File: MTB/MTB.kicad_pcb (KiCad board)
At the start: 2 copper layers, 45 parts, among them J1 BAT_CONN

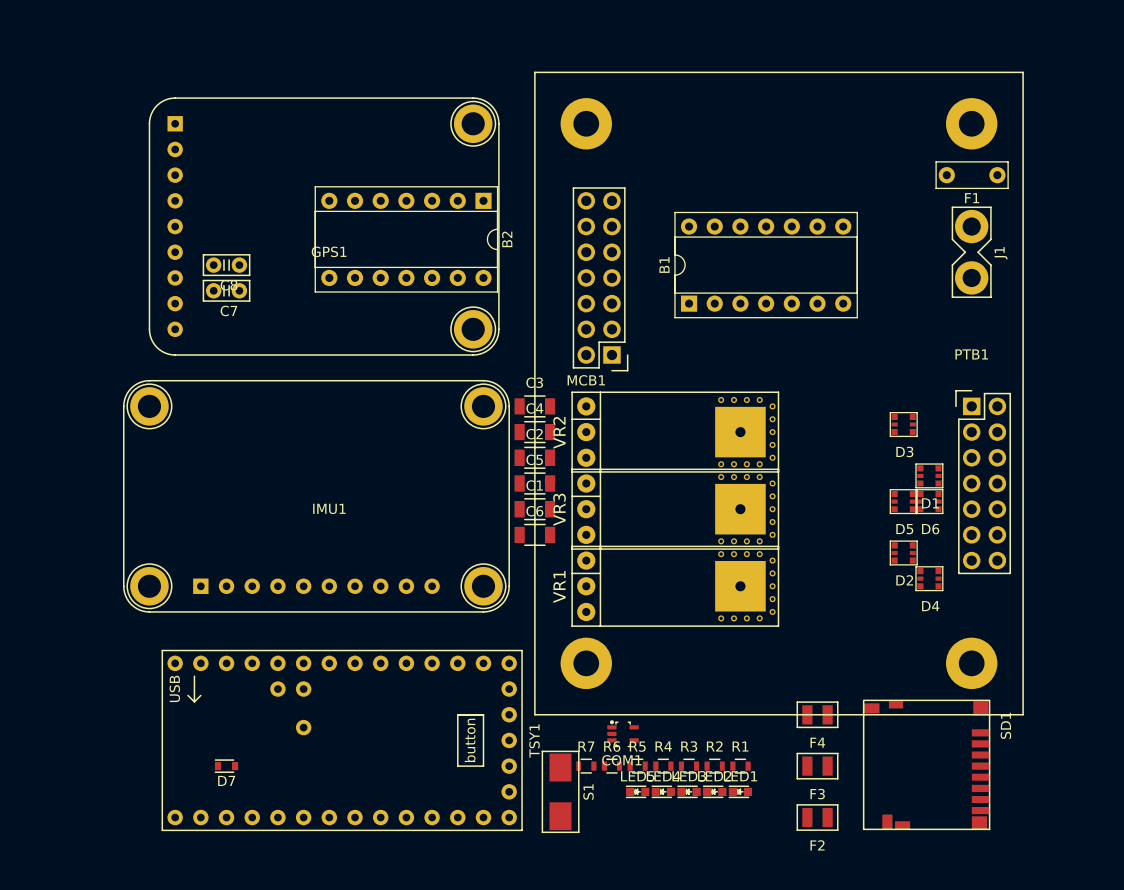
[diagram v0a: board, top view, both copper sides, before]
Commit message: finished motherboard
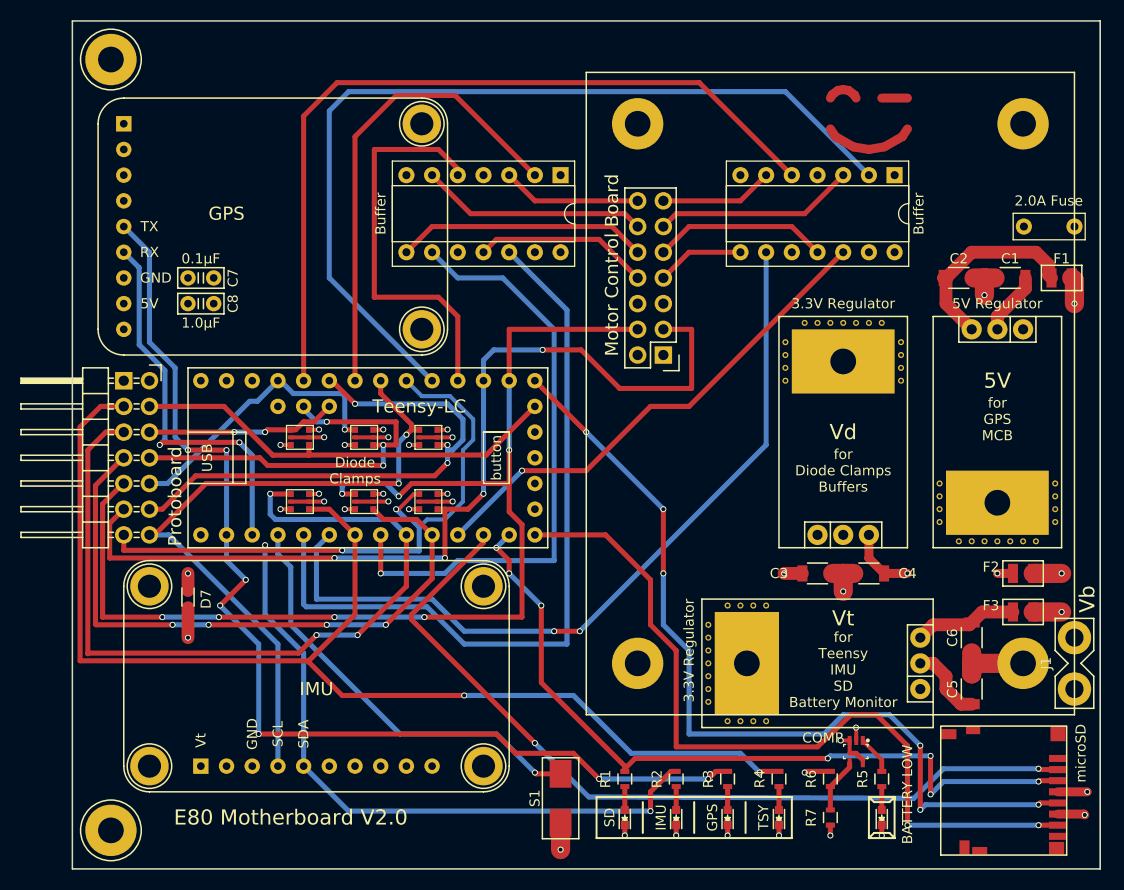
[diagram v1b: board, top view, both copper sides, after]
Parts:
- removed F4: 0.35A Fuse, MTB_footprints:1206
- removed PTB1: Protoboard, Pin_Headers:Pin_Header_Straight_2x07
- removed VR1: 5V_Regulator, MTB_footprints:VREG
- removed VR2, VR3: 3.3V_Regulator, MTB_footprints:VREG
- added 2.0A Fuse: 2.0A Fuse, Capacitors_THT:C_Disc_D7.0mm_W2.5mm_P5.00mm, F.Cu at (215.9, 83.8)
- added 3.3V Regulator: 3.3V_Regulator, MTB_footprints:VREG, F.Cu at (193.0, 114.3)
- added 3.3V Regulator: 3.3V_Regulator, MTB_footprints:VREG, F.Cu at (200.7, 127.0)
- added 5V Regulator: 5V_Regulator, MTB_footprints:VREG, F.Cu at (208.3, 94.0)
- added Protoboard: Protoboard, MTB_footprints:PTB_CONN, F.Cu at (124.5, 99.1)
- added T1: TEST_HOLE, MCB_footprints:TESTPOINT_LARGE, F.Cu at (120.7, 67.3)
- added T2: TEST_HOLE, MCB_footprints:TESTPOINT_LARGE, F.Cu at (120.7, 143.5)
- BATTERY LOW: renamed from LED5
- Buffer: renamed from B2; value Buffer -> Buffer2
- F1: value 2.0A Fuse -> .35A Fuse; footprint Capacitors_THT:C_Disc_D7.0mm_W2.5mm_P5.00mm -> MTB_footprints:1206
- F2: value 0.35A Fuse -> .35A Fuse
- F3: value 0.5A Fuse -> .5A Fuse
- Motor Control Board: renamed from MCB1
- moved D6 62.6 mm to (138.4, 105.4)
- moved D1 62.3 mm to (138.4, 111.8)
- moved D5 53.7 mm to (144.8, 105.4)
- moved D2 53.6 mm to (144.8, 111.8)
- moved C1 52.3 mm to (209.6, 88.9), turned to 180 degrees
- moved D4 51.5 mm to (151.1, 105.4)
- moved C5 47.7 mm to (205.7, 129.5), turned to 90 degrees
- moved D3 47.6 mm to (151.1, 111.8)
- moved C2 45.5 mm to (204.5, 88.9)
- moved C6 44.4 mm to (205.7, 124.5), turned to 270 degrees
- moved J1 41.9 mm to (215.9, 127.0), turned to 270 degrees
- moved Buffer 40.7 mm to (198.1, 78.7)
- moved C4 35.9 mm to (195.6, 118.1), turned to 180 degrees
- moved C3 32.5 mm to (190.5, 118.1)
- moved F2 31.5 mm to (210.8, 118.1), turned to 180 degrees
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- renumbered B1 to Buffer, COM1 to COMP, GPS1 to GPS, LED3 to GPS, IMU1 to IMU, LED2 to IMU, LED1 to SD, LED4 to TSY, TSY1 to Teensy-LC, SD1 to microSD
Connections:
- Buffer pad 14: Vt -> Vd (x2)
- Buffer pad 11: /2A -> /4A
- Buffer pad 12: 2AT -> 4AT
- Buffer pad 2: 8AT -> 6AT
- Buffer pad 3: /8A -> /6A
- Buffer pad 5: 6AT -> 8AT
- Buffer pad 6: /6A -> /8A
- Buffer pad 8: /4A -> /2A
- Buffer pad 9: 4AT -> 2AT
- C1 pad 1: Net-(C1-Pad1) -> +5V
- C2 pad 1: +5V -> Net-(C2-Pad1)
- C3 pad 1: Net-(C3-Pad1) -> Vd
- C4 pad 1: Vt -> Net-(C4-Pad1)
- C5 pad 1: Net-(C5-Pad1) -> Vt
- C6 pad 1: Vd -> Net-(C6-Pad1)
- F1 pad 1: Vm -> Vb
- F1 pad 2: Net-(F1-Pad2) -> Net-(C2-Pad1)
- F2 pad 1: Vm -> Vb
- F2 pad 2: Net-(C1-Pad1) -> Net-(C4-Pad1)
- F3 pad 1: Vm -> Vb
- F3 pad 2: Net-(C3-Pad1) -> Net-(C6-Pad1)
- J1 pad 1: Vm -> Vb
- Motor Control Board pad 3: Net-(F1-Pad2) -> Vm
- R6 pad 2: Vm -> Vb
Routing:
- net Vb: track 0.00 -> 298.3 mm, vias 0 -> 4
- net SDA0: track 0.00 -> 126.5 mm, vias 0 -> 4
- net D5: track 0.00 -> 122.0 mm, vias 0 -> 2
- net A0: track 0.00 -> 117.0 mm, vias 0 -> 7
- net RX: track 0.00 -> 108.5 mm, vias 0 -> 7
- net Vd: track 0.00 -> 93.2 mm, vias 0 -> 7
- net A1: track 0.00 -> 92.7 mm, vias 0 -> 4
- net 6AT: track 0.00 -> 88.4 mm
- net SCK0: track 0.00 -> 86.4 mm, vias 0 -> 6
- net CS0: track 0.00 -> 83.7 mm, vias 0 -> 2
- net D7: track 0.00 -> 82.1 mm, vias 0 -> 3
- net 8AT: track 0.00 -> 79.6 mm
- net 2AT: track 0.00 -> 79.3 mm, vias 0 -> 2
- net MISO0: track 0.00 -> 79.0 mm, vias 0 -> 2
- net MOSI0: track 0.00 -> 77.1 mm, vias 0 -> 7
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- added copper zone on In2.Cu, net +5V
- added copper zone on In1.Cu, net GND
- added copper zone on In2.Cu, net Vd
- added copper zone on In2.Cu, net Vt
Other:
- board outline added: 101.6 x 83.8 mm
- copper layers 2 -> 4
- net class Default: trace_width 0.25 -> 0.5
- net class High Power added: clearance 0.2, trace_width 1.9, via_dia 0.6, via_drill 0.4
- net class Power added: clearance 0.2, trace_width 1.27, via_dia 0.6, via_drill 0.4
- board text added: "(buffered)"
- board text added: "0.1µF"
- board text added: "1.0µF"
- board text added: "1A"
- board text added: "2A"
- board text added: "3A"
- board text added: "4A"
- board text added: "5A"
- board text added: "5V"
- board text added: "6A"
- board text added: "7A"
- board text added: "8A"
- board text added: "A0"
- board text added: "A1"
- board text added: "A10"
- board text added: "A11"
- board text added: "A12"
- board text added: "A7"
- board text added: "A9"
- board text added: "CS"
- board text added: "D5"
- board text added: "D7"
- board text added: "D8"
- board text added: "Diode Clamps"
- board text added: "E80 Motherboard V2.0"
- board text added: "GND"
- board text added: "MISO"
- board text added: "MOSI"
- board text added: "RX"
- board text added: "S1"
- board text added: "SCK"
- board text added: "SCL"
- board text added: "SDA"
- board text added: "TX"
- board text added: "Vb"
- board text added: "Vd"
- board text added: "Vm"
- board text added: "Vt"
- board text added: "for Diode Clamps Buffers"
- board text added: "for GPS MCB"
- board text added: "for Teensy IMU SD Battery Monitor"
